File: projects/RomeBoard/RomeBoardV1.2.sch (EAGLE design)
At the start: 38 parts, among them J2 RASPBERRY-PI-HEADER, M1 ZVN4424A, M2 ZVN4424A, M3 ZVN4424A, U1 LM1084IT-ADJ

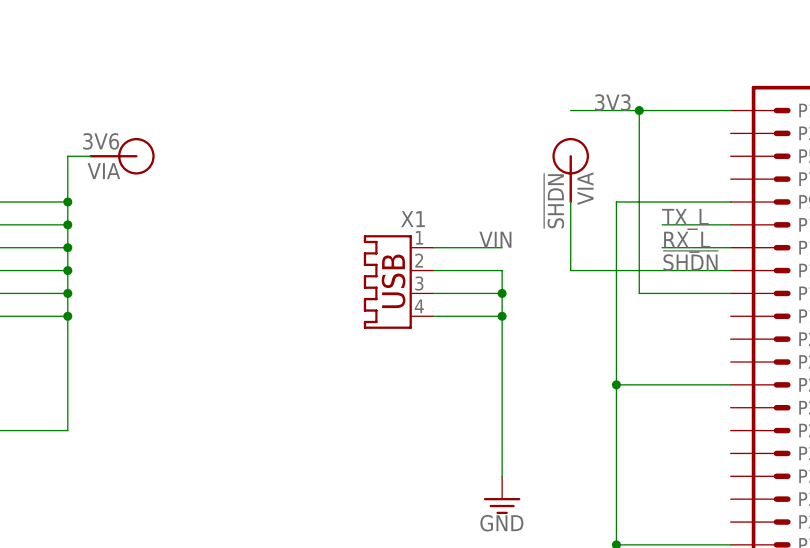
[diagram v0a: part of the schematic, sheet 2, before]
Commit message: Rome Board v1.2 updates
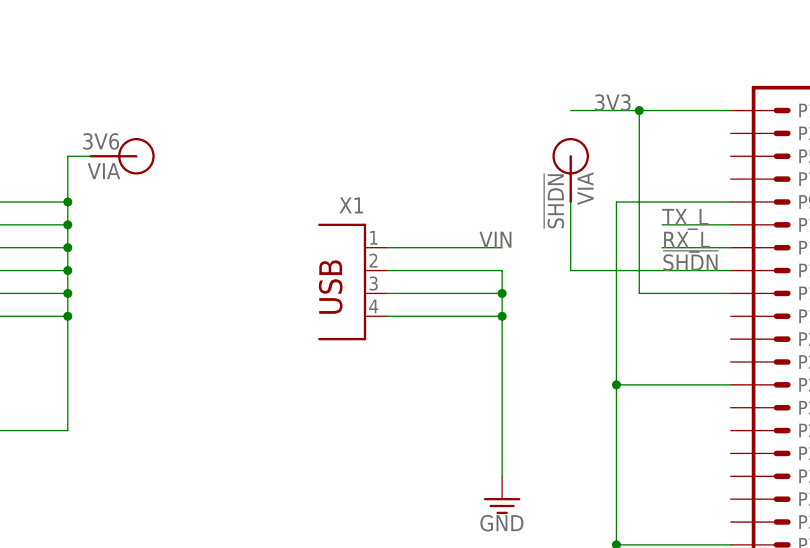
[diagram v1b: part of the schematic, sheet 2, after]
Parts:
- X1: device con-yamaichi:USB-A003 -> con-berg:PN87520
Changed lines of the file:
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@@
 <?xml version="1.0" encoding="utf-8"?>
 <!DOCTYPE eagle SYSTEM "eagle.dtd">
-<eagle version="8.3.2">
+<eagle version="9.1.0">
 <drawing>
 <settings>
@@
 <part name="V3" library="BrownSpaceEngineering" deviceset="VIA" device="-60MIL" value="GND"/>
 <part name="V6" library="BrownSpaceEngineering" deviceset="VIA" device="-60MIL" value="!SHDN"/>
-<part name="X1" library="con-yamaichi" library_urn="urn:adsk.eagle:library:202" deviceset="USB-A003" device="" package3d_urn="urn:adsk.eagle:package:11805/1"/>
+<part name="X1" library="con-berg" library_urn="urn:adsk.eagle:library:130" deviceset="PN87520" device="" package3d_urn="urn:adsk.eagle:package:6146/1"/>
 </parts>
 <sheets>
@@
 <instance part="V3" gate="G$1" x="264.16" y="30.48" rot="R180"/>
 <instance part="V6" gate="G$1" x="190.5" y="45.72" rot="R270"/>
-<instance part="X1" gate="G$1" x="170.18" y="30.48" rot="MR0"/>
+<instance part="X1" gate="G$1" x="167.64" y="30.48" rot="MR0"/>
 </instances>
 <busses>
@@
 <pinref part="GND3" gate="1" pin="GND"/>
 <wire x1="182.88" y1="10.16" x2="182.88" y2="27.94" width="0.1524" layer="91"/>
-<wire x1="175.26" y1="27.94" x2="182.88" y2="27.94" width="0.1524" layer="91"/>
-<wire x1="175.26" y1="30.48" x2="182.88" y2="30.48" width="0.1524" layer="91"/>
 <wire x1="182.88" y1="27.94" x2="182.88" y2="30.48" width="0.1524" layer="91"/>
 <junction x="182.88" y="27.94"/>
-<wire x1="175.26" y1="33.02" x2="182.88" y2="33.02" width="0.1524" layer="91"/>
 <wire x1="182.88" y1="30.48" x2="182.88" y2="33.02" width="0.1524" layer="91"/>
 <junction x="182.88" y="30.48"/>
 <pinref part="X1" gate="G$1" pin="2"/>
+<wire x1="170.18" y1="33.02" x2="182.88" y2="33.02" width="0.1524" layer="91"/>
 <pinref part="X1" gate="G$1" pin="3"/>
+<wire x1="182.88" y1="30.48" x2="170.18" y2="30.48" width="0.1524" layer="91"/>
 <pinref part="X1" gate="G$1" pin="4"/>
+<wire x1="170.18" y1="27.94" x2="182.88" y2="27.94" width="0.1524" layer="91"/>
 </segment>
 <segment>
@@
 <net name="VIN" class="0">
 <segment>
-<wire x1="175.26" y1="35.56" x2="182.88" y2="35.56" width="0.1524" layer="91"/>
 <label x="180.34" y="35.56" size="1.778" layer="95"/>
 <pinref part="X1" gate="G$1" pin="1"/>
-</segment>
-</net>
+<wire x1="182.88" y1="35.56" x2="170.18" y2="35.56" width="0.1524" layer="91"/>
+</segment>
+</net>
